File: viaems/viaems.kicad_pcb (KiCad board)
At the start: 2 copper layers, 136 x 64 mm, 210 parts, among them J1 Conn_02x08_Counter_Clockwise, J10 Conn_01x04, J11 Conn_01x08, J12 Conn_01x02, J13 Conn_01x06, J14 Conn_01x06, J15 Conn_02x06_Odd_Even, J16 VBAT, J17 Conn_01x04, J18 USB_B_Micro, J19 Conn_ARM_JTAG_SWD_10, J2 Conn_01x02, J20 SPI, J21 Conn_01x02, J3 Conn_01x03, J4 Conn_01x04, J5 Conn_01x02, J6 Conn_01x02, J7 Conn_01x04, J8 Conn_01x04, J9 Conn_01x08, Q1 VND7NV04, Q2 VND7NV04, Q3 VND7NV04, Q4 VND7NV04, Q5 VND7NV04, Q6 VND7NV04, Q7 VND7NV04, Q8 VND7NV04, U1 LM2940, U10 MCP2562-H-SN, U11 NCP1117-3.3_TO252, U12 MPXH6400A, U13 MPXH6115AC6U, U14 MAX9926UAEE+, U15 LM2940, U16 AD7888, U2 TC442xA, U3 TC442xA, U4 TC442xA, U5 TC442xA, U6 TC442xA, U7 TC442xA, U8 TC442xA, U9 STM32F407VGTx, Y1 8 Mhz

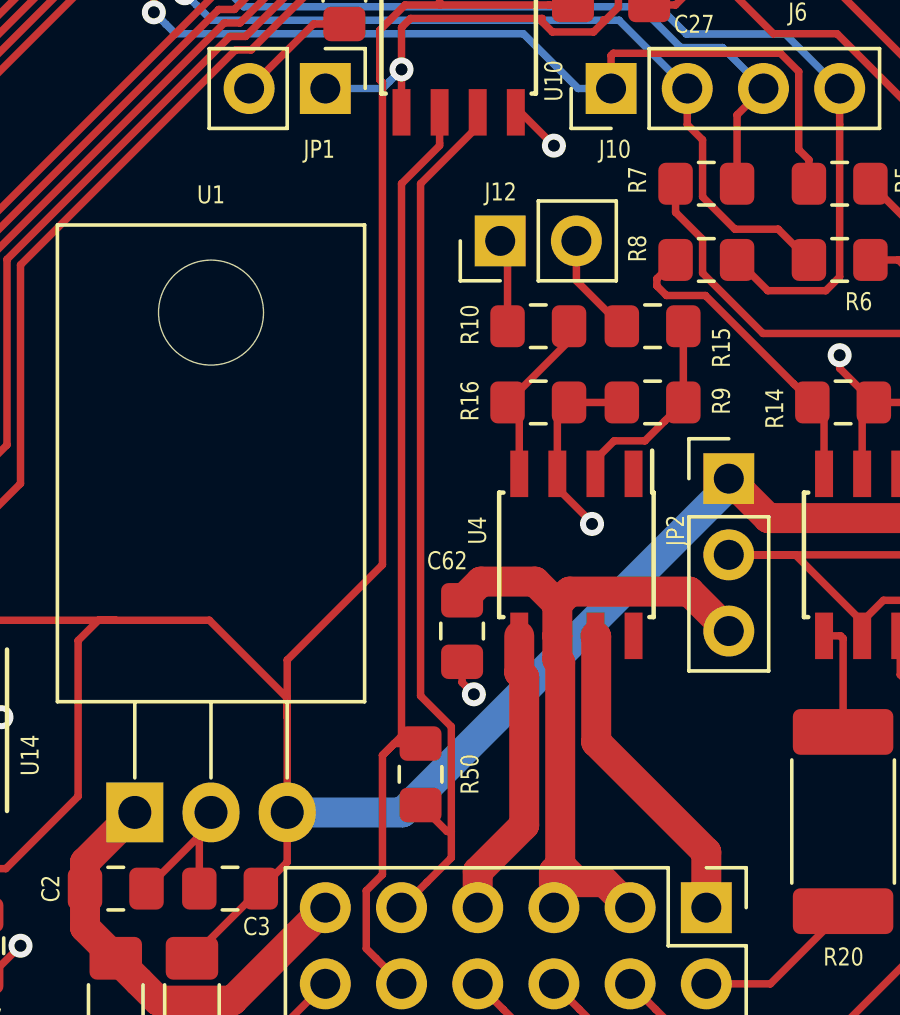
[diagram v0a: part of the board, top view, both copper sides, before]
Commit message: Misc fixes
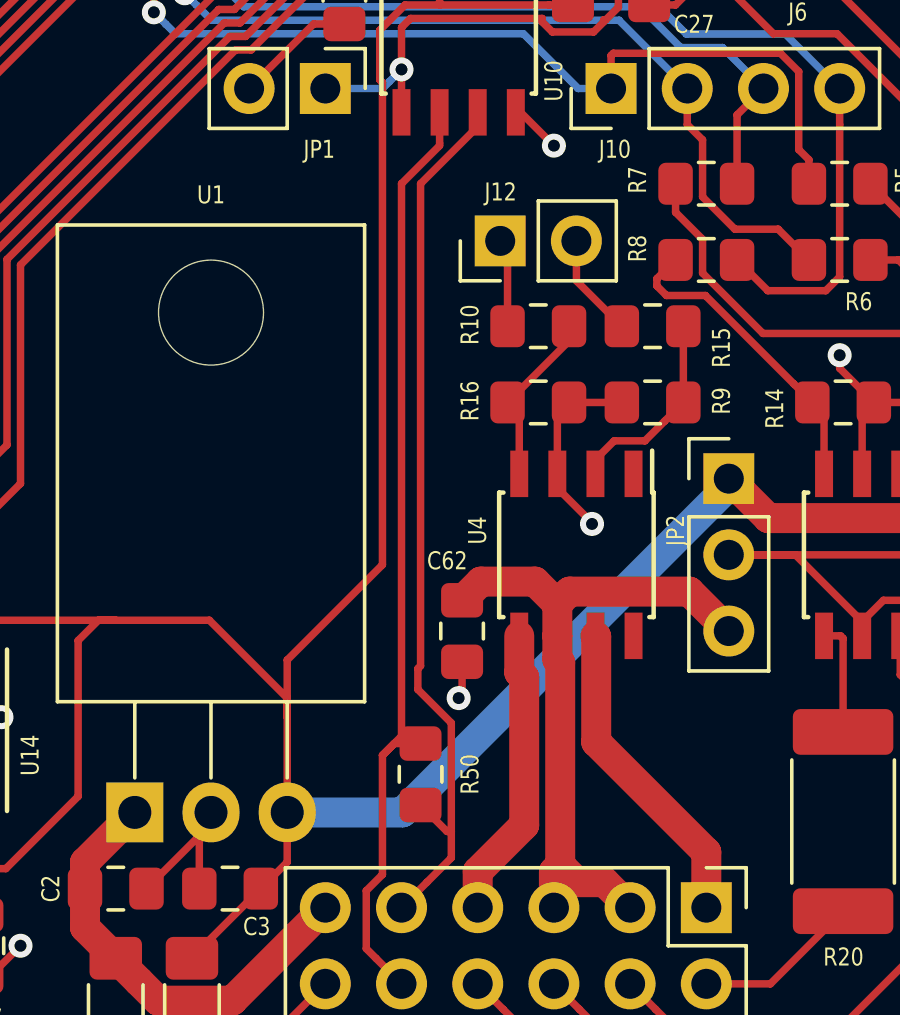
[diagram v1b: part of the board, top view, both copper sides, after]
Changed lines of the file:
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@@
-(kicad_pcb (version 20171130) (host pcbnew 5.0.1+dfsg1-3~bpo9+1)
+(kicad_pcb (version 20171130) (host pcbnew 5.0.2+dfsg1-1)
   (general
     (thickness 1.6)
     (drawings 10)
-    (tracks 1998)
+    (tracks 2000)
     (zones 0)
     (modules 210)
@@
     (34 B.Paste user hide)
     (35 F.Paste user hide)
-    (36 B.SilkS user hide)
-    (37 F.SilkS user)
+    (36 B.SilkS user)
+    (37 F.SilkS user hide)
     (38 B.Mask user hide)
     (39 F.Mask user hide)
@@
   (segment (start 139.655 90.76) (end 140.335 91.44) (width 0.25) (layer F.Cu) (net 1))
   (segment (start 139.655 90.17) (end 139.655 90.76) (width 0.25) (layer F.Cu) (net 1))
-  (segment (start 115.0493 127.7493) (end 115.442224 128.142224) (width 0.25) (layer F.Cu) (net 1))
-  (segment (start 115.0493 127.0598) (end 115.0493 127.7493) (width 0.25) (layer F.Cu) (net 1))
-  (via (at 115.442224 128.142224) (size 0.8) (drill 0.4) (layers F.Cu B.Cu) (net 1))
   (segment (start 143.381295 119.505944) (end 142.981296 119.905943) (width 0.25) (layer F.Cu) (net 1))
   (segment (start 144.193156 119.505944) (end 143.381295 119.505944) (width 0.25) (layer F.Cu) (net 1))
@@
   (segment (start 155.365 89.325) (end 154.94 88.9) (width 1) (layer F.Cu) (net 1))
   (segment (start 157.105 89.325) (end 155.365 89.325) (width 1) (layer F.Cu) (net 1))
+  (segment (start 115.0493 127.0598) (end 115.0493 128.15571) (width 0.25) (layer F.Cu) (net 1))
+  (segment (start 115.0493 128.15571) (end 114.935 128.27001) (width 0.25) (layer F.Cu) (net 1))
+  (via (at 114.935 128.27001) (size 0.8) (drill 0.4) (layers F.Cu B.Cu) (net 1))
   (segment (start 104.276347 137.713847) (end 103.505 136.9425) (width 1) (layer F.Cu) (net 2))
   (segment (start 107.38999 138.35501) (end 104.91751 138.35501) (width 1) (layer F.Cu) (net 2))
@@
   (segment (start 113.665 131.835) (end 114.545 132.715) (width 0.25) (layer F.Cu) (net 99))
   (segment (start 114.545 132.715) (end 114.69001 132.715) (width 0.25) (layer F.Cu) (net 99))
-  (segment (start 113.665 111.125) (end 113.665 128.19681) (width 0.25) (layer F.Cu) (net 99))
-  (segment (start 114.69001 129.22182) (end 114.69001 132.715) (width 0.25) (layer F.Cu) (net 99))
   (segment (start 115.57 108.745) (end 115.57 109.22) (width 0.25) (layer F.Cu) (net 99))
   (segment (start 115.57 109.22) (end 113.665 111.125) (width 0.25) (layer F.Cu) (net 99))
-  (segment (start 113.665 128.19681) (end 114.69001 129.22182) (width 0.25) (layer F.Cu) (net 99))
+  (segment (start 113.57499 127.286998) (end 113.57499 127.982998) (width 0.25) (layer F.Cu) (net 99))
+  (segment (start 113.57499 127.982998) (end 114.69001 129.098018) (width 0.25) (layer F.Cu) (net 99))
+  (segment (start 113.665 111.125) (end 113.665 127.196988) (width 0.25) (layer F.Cu) (net 99))
+  (segment (start 114.69001 129.098018) (end 114.69001 132.715) (width 0.25) (layer F.Cu) (net 99))
+  (segment (start 113.665 127.196988) (end 113.57499 127.286998) (width 0.25) (layer F.Cu) (net 99))
   (segment (start 116.419999 138.644999) (end 115.57 137.795) (width 0.25) (layer F.Cu) (net 100))
   (segment (start 117.925011 140.150011) (end 116.419999 138.644999) (width 0.25) (layer F.Cu) (net 100))
